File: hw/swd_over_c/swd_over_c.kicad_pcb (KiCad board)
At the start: 4 copper layers, 20.5 x 10.5 mm, 17 parts, among them J1 USB_C_Receptacle_USB2.0, J2 Conn_ARM_JTAG_SWD_10, P1 USB_C_Plug, U1 ATtiny24-20M

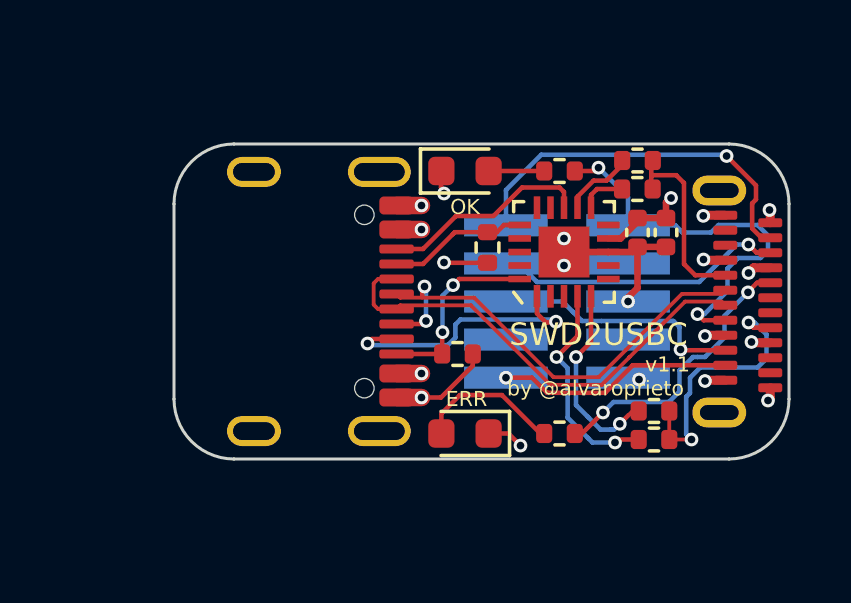
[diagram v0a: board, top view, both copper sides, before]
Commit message: SWD2USBC v1.2
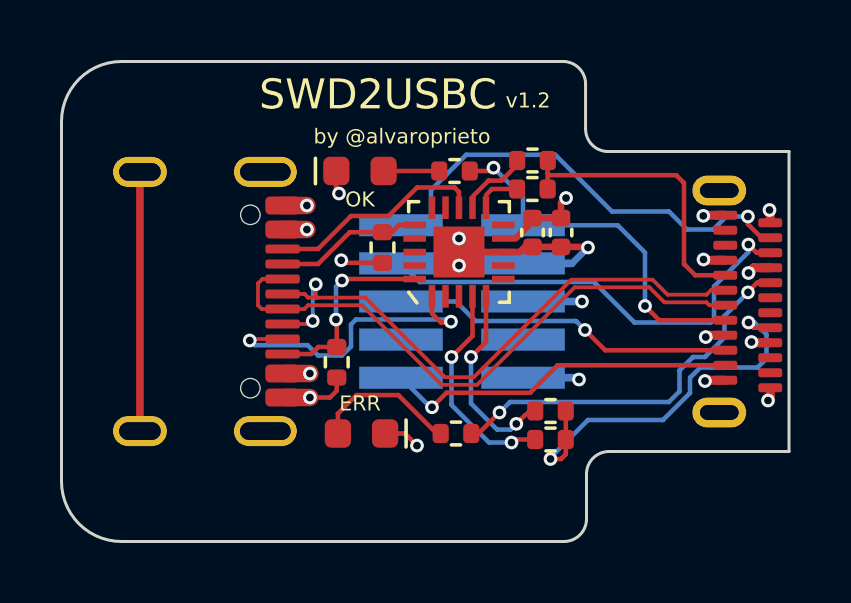
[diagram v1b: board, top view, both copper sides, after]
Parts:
- moved REF** 4.30 mm to (158.5, 67.5)
- moved R1 4.03 mm to (164.4, 69.5), turned to 90 degrees
- moved J1 3.80 mm to (162.6, 67.5)
- moved C1 3.50 mm to (170.9, 65.2)
- moved C2 3.50 mm to (171.9, 65.2)
- moved D1 3.50 mm to (165.2, 63.1)
- moved J2 3.50 mm to (168.6, 67.5)
- moved R2 3.50 mm to (165.9, 65.7)
- moved R3 3.50 mm to (170.9, 63.8)
- moved R4 3.50 mm to (170.9, 62.8)
- moved R7 3.50 mm to (168.3, 63.1)
- moved U1 3.50 mm to (168.5, 65.8)
- moved D2 3.45 mm to (165.2, 71.9)
- moved R5 3.45 mm to (171.6, 72.1)
- moved R6 3.45 mm to (171.6, 71.2)
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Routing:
- net /SHIELD: track 41.4 -> 52.0 mm
- net /SWDCLK: track 9.70 -> 15.1 mm
- net /D+: track 15.9 -> 20.3 mm
- net /D-: track 15.7 -> 20.0 mm
- net /CC2: track 9.05 -> 13.3 mm
- net /NRST: track 7.90 -> 11.8 mm
- net /CC1: track 6.37 -> 9.86 mm
- net /SBU2: track 9.44 -> 12.6 mm
- net /SWO: track 8.40 -> 11.5 mm
- net /SWDIO: track 12.6 -> 14.6 mm
- net GND: track 18.0 -> 19.4 mm, vias 13 -> 14
- net /SBU1: track 13.4 -> 12.1 mm
- net /SCK: track 9.32 -> 10.3 mm
- net VBUS: track 7.69 -> 6.80 mm
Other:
- board size 20.5 x 10.5 mm -> 24.2 x 16 mm
- board text added: "v1.2"
- board text removed: "v1.1"
